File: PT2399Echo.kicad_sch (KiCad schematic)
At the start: 85 parts, among them Q21 2N3904, Q22 2N3904, Q23 2N3906, Q24 2N3906, SW47 SW_DPDT_x2, U28 TL074, U29 TL074, U30 LM13700, U31 PT2399

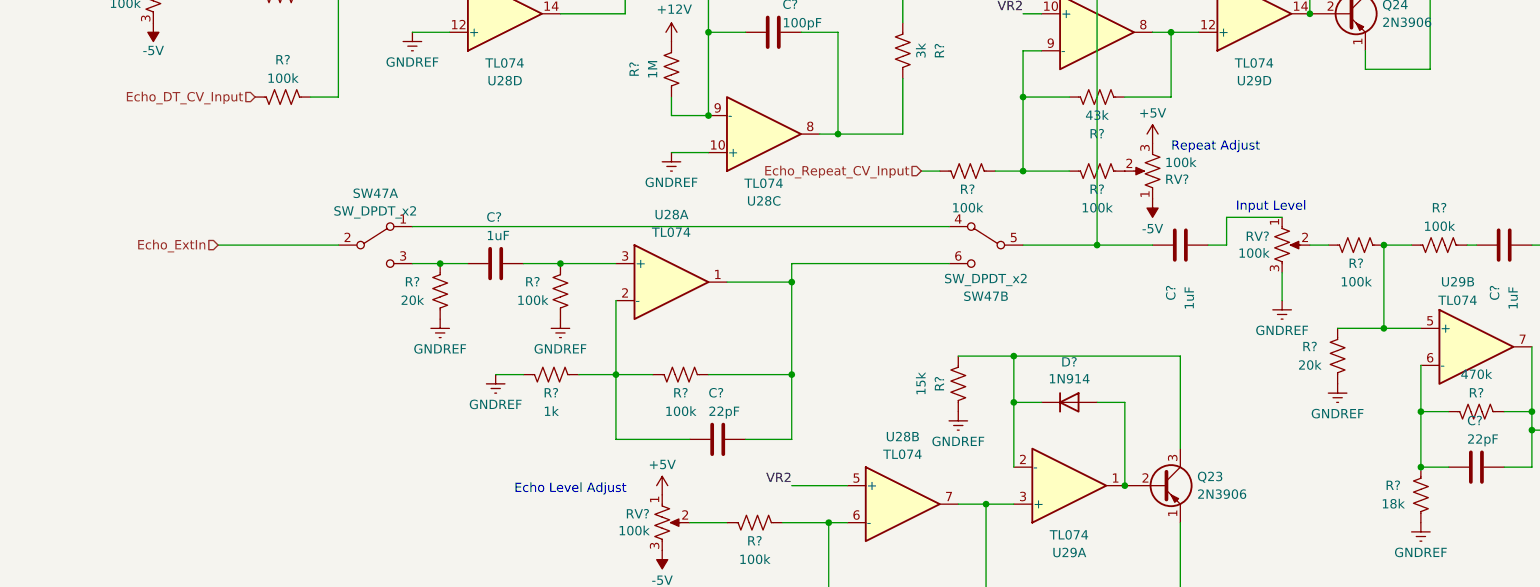
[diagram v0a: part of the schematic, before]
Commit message: routing work...
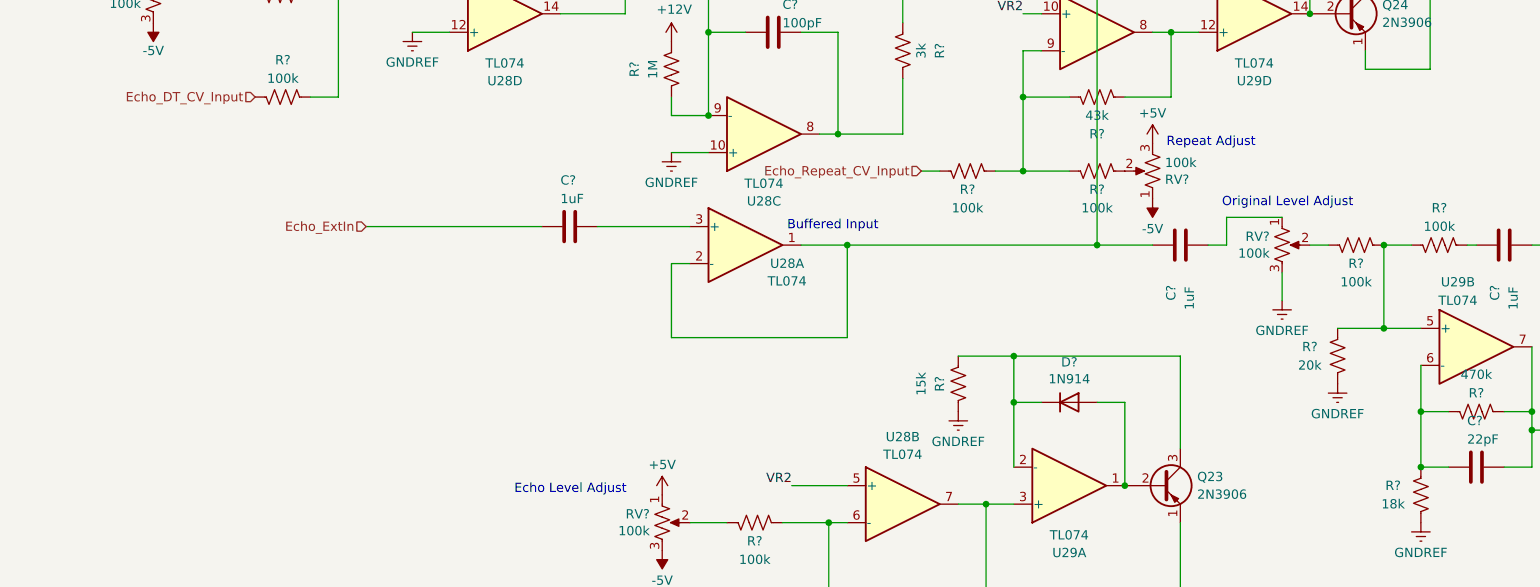
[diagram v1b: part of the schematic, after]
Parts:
- removed C?: 22pF, Capacitor_SMD:C_0603_1608Metric, symbol Device:C
- removed R? (x2): 100k, Resistor_SMD:R_0603_1608Metric, symbol Device:R_US
- removed R?: 1k, Resistor_SMD:R_0603_1608Metric, symbol Device:R_US
- removed R?: 20k, Resistor_SMD:R_0603_1608Metric, symbol Device:R_US
- removed SW47: SW_DPDT_x2, SynthProjConnectors:MTS-203-A1-T0, symbol Switch:SW_DPDT_x2
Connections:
- net Echo_ExtIn: now also C?.2
- net at U28.2 (-): now also C?.1, C?.1, U28.1
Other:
- note added: "Buffered Input"
- note added: "Original Level Adjust"
- note removed: "Input Level"
- moved on the sheet: C?, U28A

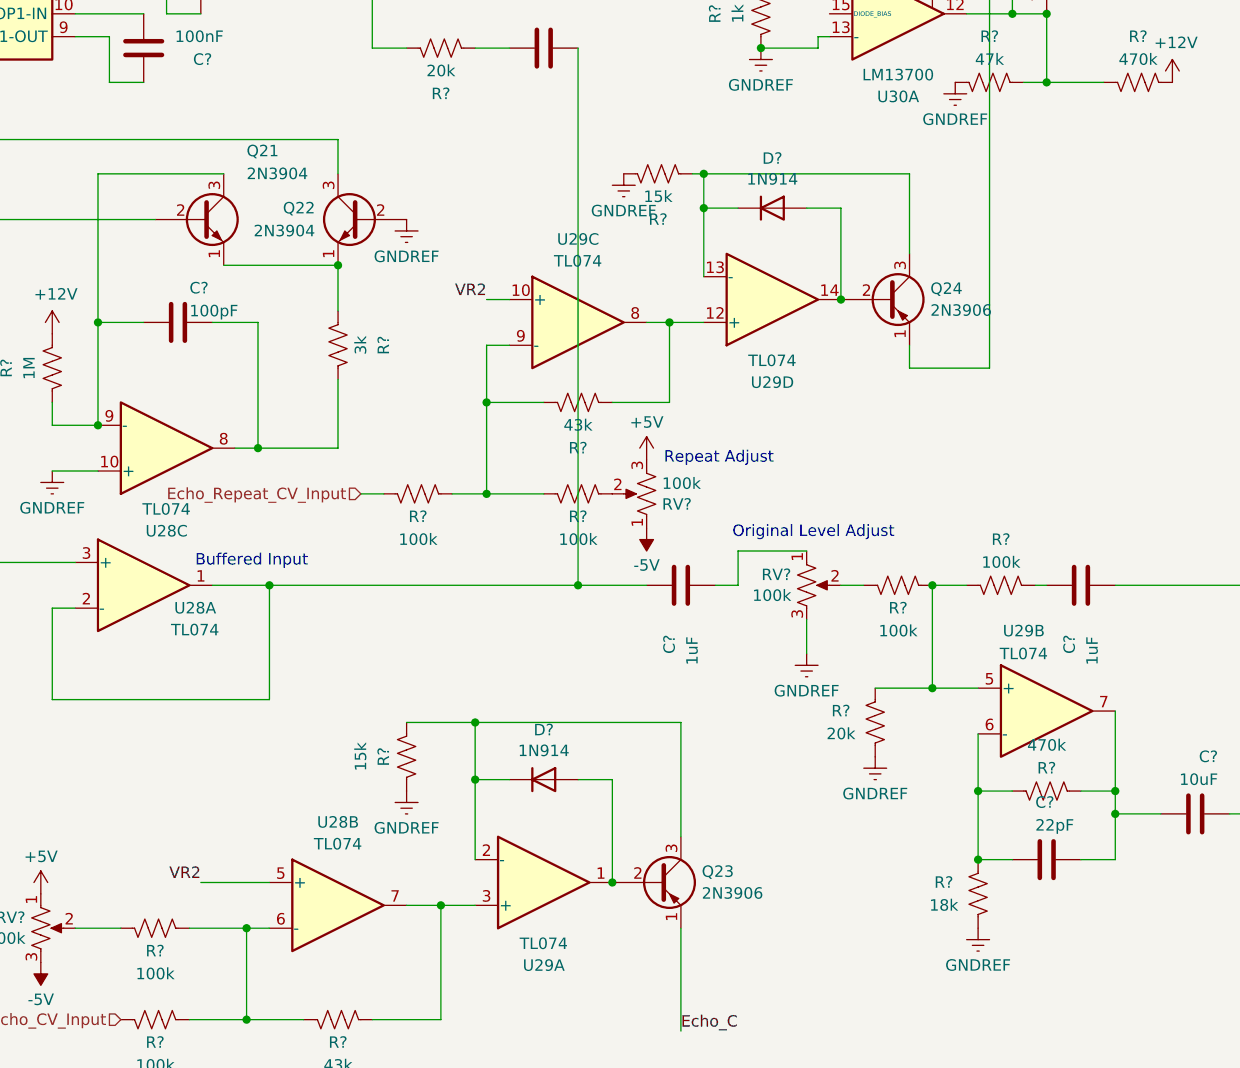
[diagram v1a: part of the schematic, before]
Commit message: routing... placing... going cross eyed...
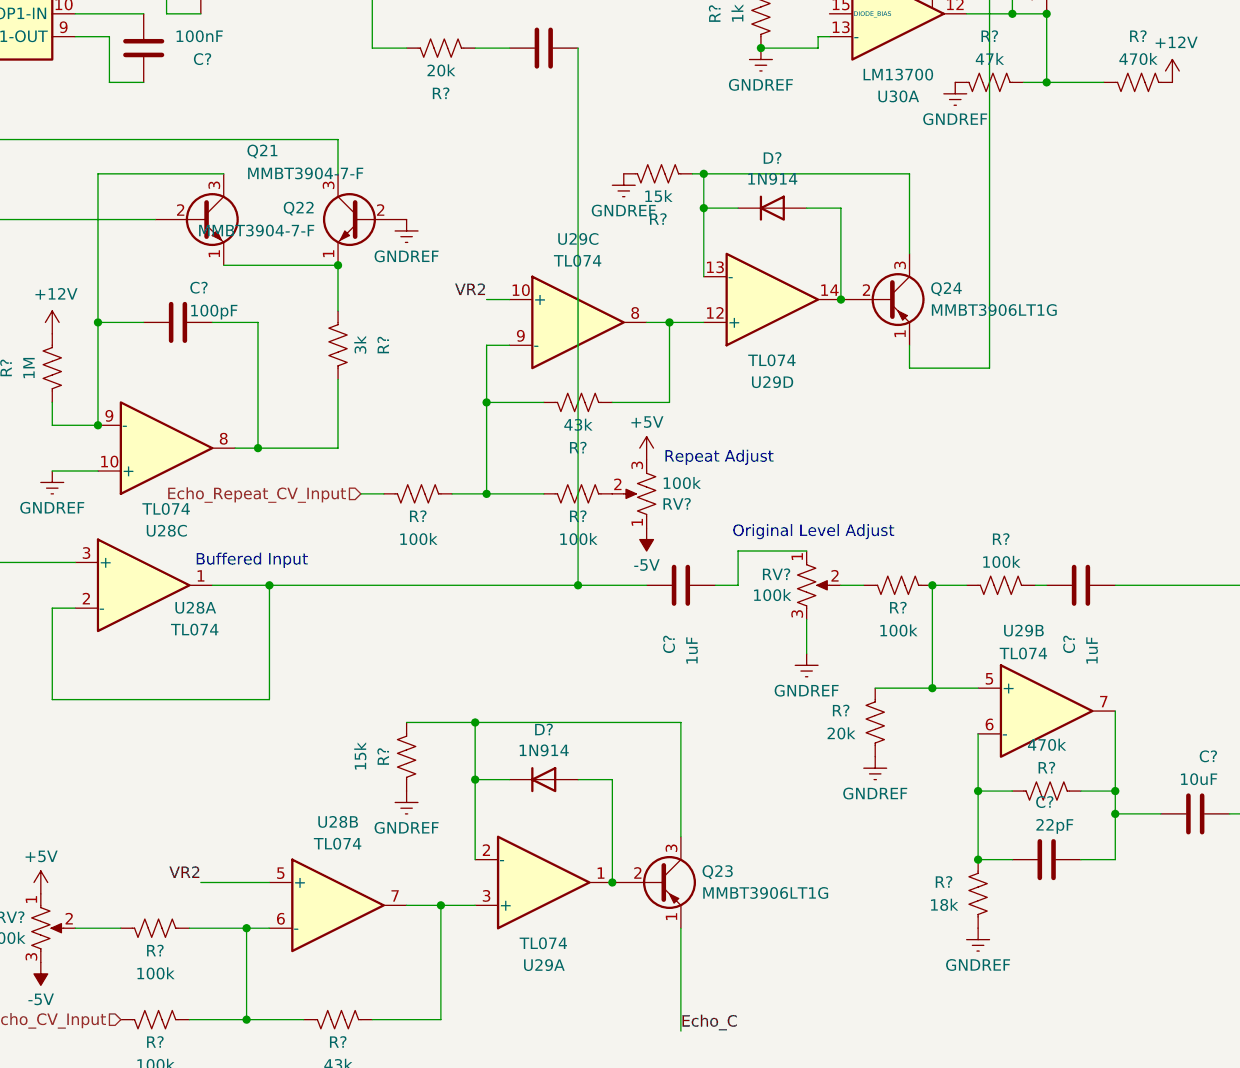
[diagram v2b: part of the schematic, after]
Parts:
- Q21, Q22: value 2N3904 -> MMBT3904-7-F; footprint Package_TO_SOT_THT:TO-92_Inline -> Package_TO_SOT_SMD:SOT-23-3
- Q23, Q24: value 2N3906 -> MMBT3906LT1G; footprint Package_TO_SOT_THT:TO-92_Inline -> Package_TO_SOT_SMD:SOT-23-3
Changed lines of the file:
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@@
       (effects (font (size 1.27 1.27)) (justify left))
     )
-    (property "Value" "2N3906" (at 200.4314 90.1121 0)
+    (property "Value" "MMBT3906LT1G" (at 200.4314 90.1121 0)
       (effects (font (size 1.27 1.27)) (justify left))
     )
-    (property "Footprint" "Package_TO_SOT_THT:TO-92_Inline" (at 200.66 90.805 0)
+    (property "Footprint" "Package_TO_SOT_SMD:SOT-23-3" (at 200.66 90.805 0)
       (effects (font (size 1.27 1.27) italic) (justify left) hide)
     )
@@
       (effects (font (size 1.27 1.27)) (justify left))
     )
-    (property "Value" "2N3904" (at 132.08 81.28 0)
+    (property "Value" "MMBT3904-7-F" (at 132.08 81.28 0)
       (effects (font (size 1.27 1.27)) (justify left))
     )
-    (property "Footprint" "Package_TO_SOT_THT:TO-92_Inline" (at 132.08 81.915 0)
+    (property "Footprint" "Package_TO_SOT_SMD:SOT-23-3" (at 132.08 81.915 0)
       (effects (font (size 1.27 1.27) italic) (justify left) hide)
     )
@@
       (effects (font (size 1.27 1.27)) (justify left))
     )
-    (property "Value" "2N3904" (at 124.46 74.93 0)
+    (property "Value" "MMBT3904-7-F" (at 124.46 74.93 0)
       (effects (font (size 1.27 1.27)) (justify left))
     )
-    (property "Footprint" "Package_TO_SOT_THT:TO-92_Inline" (at 124.46 81.915 0)
+    (property "Footprint" "Package_TO_SOT_SMD:SOT-23-3" (at 124.46 81.915 0)
       (effects (font (size 1.27 1.27) italic) (justify left) hide)
     )
@@
       (effects (font (size 1.27 1.27)) (justify left))
     )
-    (property "Value" "2N3906" (at 175.0314 154.8821 0)
+    (property "Value" "MMBT3906LT1G" (at 175.0314 154.8821 0)
       (effects (font (size 1.27 1.27)) (justify left))
     )
-    (property "Footprint" "Package_TO_SOT_THT:TO-92_Inline" (at 175.26 155.575 0)
+    (property "Footprint" "Package_TO_SOT_SMD:SOT-23-3" (at 175.26 155.575 0)
       (effects (font (size 1.27 1.27) italic) (justify left) hide)
     )

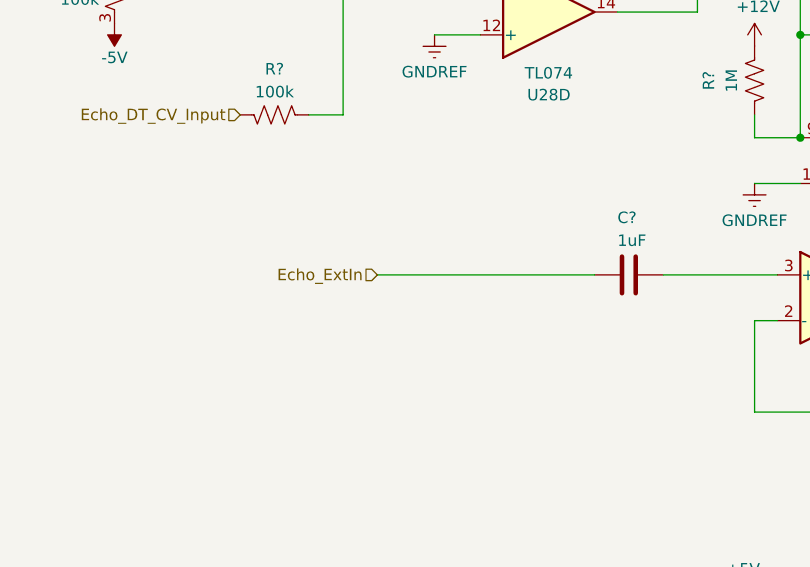
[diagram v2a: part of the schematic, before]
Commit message: more and more routing
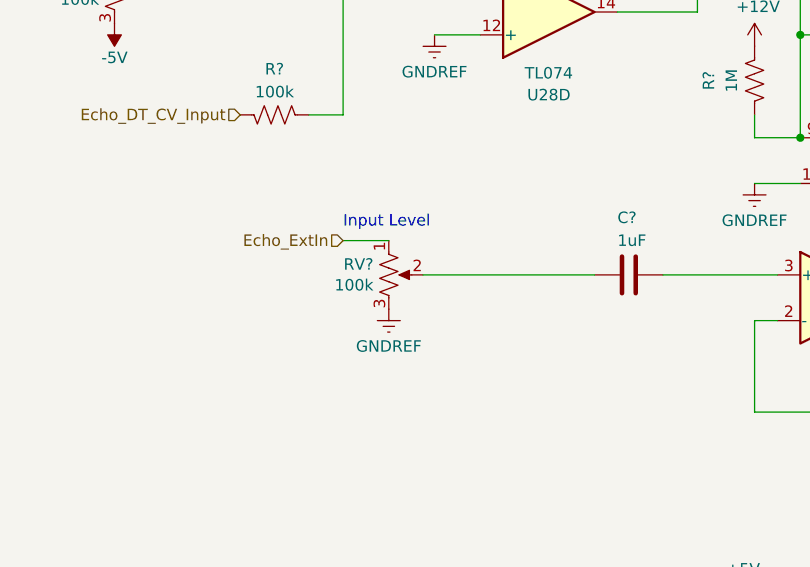
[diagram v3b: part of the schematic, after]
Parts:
- added RV?: 100k, Potentiometer_THT:Potentiometer_Alps_RK09K_Single_Vertical, symbol SynthProj-rescue:R_POT_US-Device
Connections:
- net Echo_ExtIn: now also RV?.1; no longer C?.2
- net GNDREF: now also RV?.3
- new net: C?.2, RV?.2
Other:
- note added: "Input Level"
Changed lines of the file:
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@@
     (stroke (width 0) (type default))
   )
+  (wire (pts (xy 57.15 114.3) (xy 62.23 114.3))
+    (stroke (width 0) (type default))
+  )
   (wire (pts (xy 179.07 120.65) (xy 179.07 116.84))
     (stroke (width 0) (type default))
@@
     (stroke (width 0) (type default))
   )
+  (wire (pts (xy 66.04 118.11) (xy 85.09 118.11))
+    (stroke (width 0) (type default))
+  )
   (wire (pts (xy 236.22 22.86) (xy 236.22 33.02))
     (stroke (width 0) (type default))
@@
     (stroke (width 0) (type default))
   )
-  (wire (pts (xy 60.96 118.11) (xy 85.09 118.11))
-    (stroke (width 0) (type default))
-  )
   (wire (pts (xy 69.85 86.36) (xy 72.39 86.36))
     (stroke (width 0) (type default))
@@
     (effects (font (size 1.27 1.27)) (justify left bottom))
   )
+  (text "Input Level" (at 57.15 113.03 0)
+    (effects (font (size 1.27 1.27)) (justify left bottom))
+  )
   (text "Delay Time Adjust" (at 12.7 81.28 0)
     (effects (font (size 1.27 1.27)) (justify left bottom))
@@
     (effects (font (size 1.27 1.27)) (justify right))
   )
-  (hierarchical_label "Echo_ExtIn" (shape input) (at 60.96 118.11 180) (fields_autoplaced)
+  (hierarchical_label "Echo_ExtIn" (shape input) (at 57.15 114.3 180) (fields_autoplaced)
     (effects (font (size 1.27 1.27)) (justify right))
   )
@@
     )
   )
+  (symbol (lib_id "power:GNDREF") (at 62.23 121.92 0) (mirror y) (unit 1)
+    (in_bom yes) (on_board yes) (dnp no) (fields_autoplaced)
+    (property "Reference" "#PWR0273" (at 62.23 128.27 0)
+      (effects (font (size 1.27 1.27)) hide)
+    )
+    (property "Value" "GNDREF" (at 62.23 126.0531 0)
+      (effects (font (size 1.27 1.27)))
+    )
+    (property "Footprint" "" (at 62.23 121.92 0)
+      (effects (font (size 1.27 1.27)) hide)
+    )
+    (property "Datasheet" "" (at 62.23 121.92 0)
+      (effects (font (size 1.27 1.27)) hide)
+    )
+    (pin "1")
+    (instances
+      (project "SynthProj"
+        (path "/9021c97e-351f-4ed9-b393-50257df6a463/0e948a88-c071-4754-aa3e-af223f738530"
+          (reference "#PWR0273") (unit 1)
+        )
+      )
+    )
+  )
   (symbol (lib_id "Transistor_BJT:2N3906") (at 195.58 88.9 0) (unit 1)
     (in_bom yes) (on_board yes) (dnp no)
@@
         )
       )
+    )
+  )
+  (symbol (lib_id "SynthProj-rescue:R_POT_US-Device") (at 62.23 118.11 0) (unit 1)
+    (in_bom yes) (on_board yes) (dnp no)
+    (property "Reference" "RV?" (at 60.5282 116.9416 0)
+      (effects (font (size 1.27 1.27)) (justify right))
+    )
+    (property "Value" "100k" (at 60.5282 119.253 0)
+      (effects (font (size 1.27 1.27)) (justify right))
+    )
+    (property "Footprint" "Potentiometer_THT:Potentiometer_Alps_RK09K_Single_Vertical" (at 62.23 118.11 0)
+      (effects (font (size 1.27 1.27)) hide)
+    )
+    (property "Datasheet" "~" (at 62.23 118.11 0)
+      (effects (font (size 1.27 1.27)) hide)
+    )
+    (pin "2")
+    (pin "3")
+    (pin "1")
+    (instances
+      (project "SynthProj"
+        (path "/9021c97e-351f-4ed9-b393-50257df6a463/00000000-0000-0000-0000-0000659d0967"
+          (reference "RV?") (unit 1)
+        )
+        (path "/9021c97e-351f-4ed9-b393-50257df6a463/00000000-0000-0000-0000-0000659a4e2e"
+          (reference "RV?") (unit 1)
+        )
+        (path "/9021c97e-351f-4ed9-b393-50257df6a463"
+          (reference "RV?") (unit 1)
+        )
+        (path "/9021c97e-351f-4ed9-b393-50257df6a463/0e948a88-c071-4754-aa3e-af223f738530"
+          (reference "RV51") (unit 1)
+        )
+      )

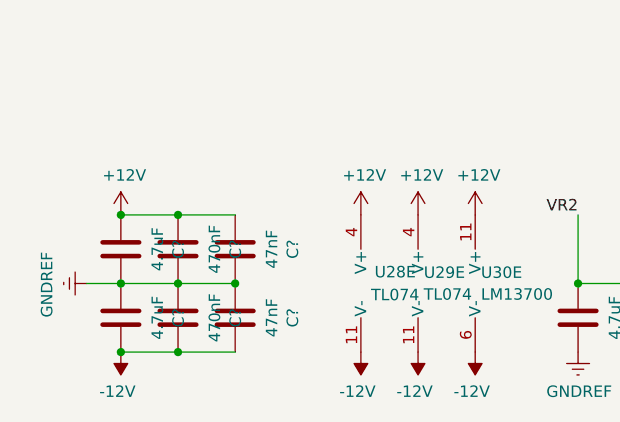
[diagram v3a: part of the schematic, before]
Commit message: more and more and more and more and more routing
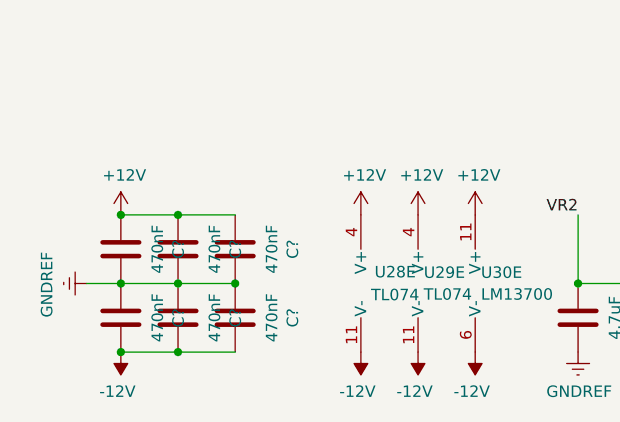
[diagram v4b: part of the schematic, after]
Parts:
- removed C? (x2): 4.7uF, Capacitor_SMD:C_0805_2012Metric, symbol Device:C
- removed C? (x2): 47nF, Capacitor_SMD:C_0603_1608Metric, symbol Device:C
- added C? (x4): 470nF, Capacitor_SMD:C_0805_2012Metric, symbol Device:C
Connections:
- net +12V: now also C?.2, C?.2
- net -12V: now also C?.1, C?.1
- net GNDREF: now also C?.1, C?.1, C?.2, C?.2
